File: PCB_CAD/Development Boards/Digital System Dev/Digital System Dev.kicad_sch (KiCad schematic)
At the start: 73 parts, among them J1 STLINK, J10 10V, J2 PINS_LEFT, J3 3V3, J4 5V, J5 GND, J6 PINS_LEFT, J7 DISP, J9 DC_IN, SW1 RESET, U1 STM32G474VETx, U2 DFR0570, U3 DFR0571, X1 HSE_24

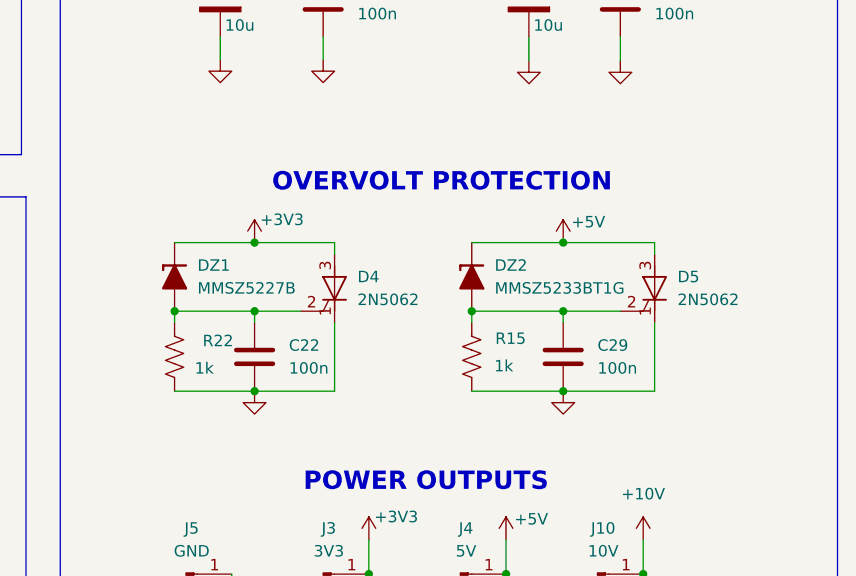
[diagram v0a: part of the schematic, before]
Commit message: fix num 2 for my cpu hungry i2c scheduler :c
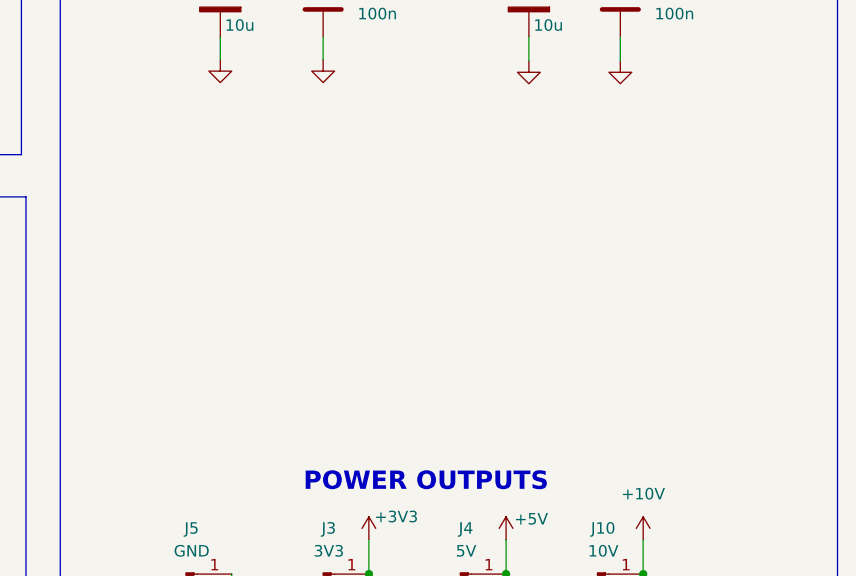
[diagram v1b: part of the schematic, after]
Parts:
- removed C22, C29: 100n, Capacitor_SMD:C_0603_1608Metric, symbol Device:C
- removed D4, D5: 2N5062, Package_TO_SOT_THT:TO-92, symbol Device:Q_SCR_KGA
- removed DZ1: MMSZ5227B, Diode_SMD:D_SOD-123, symbol PCM_Diode_Zener_AKL:D_Zener_Generic
- removed DZ2: MMSZ5233BT1G, Diode_SMD:D_SOD-123, symbol PCM_Diode_Zener_AKL:D_Zener_Generic
- removed R15, R22: 1k, Resistor_SMD:R_0603_1608Metric, symbol Device:R_US
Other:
- note removed: "OVERVOLT PROTECTION"
